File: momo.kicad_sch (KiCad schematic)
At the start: 97 parts, among them SW1 MX_SW_HS, SW10 MX_SW_HS, SW11 MX_SW_HS, SW12 MX_SW_HS, SW13 MX_SW_HS, SW14 MX_SW_HS, SW15 MX_SW_HS, SW16 MX_SW_HS, SW17 MX_SW_HS, SW18 MX_SW_HS, SW19 MX_SW_HS, SW2 MX_SW_HS, SW20 MX_SW_HS, SW21 MX_SW_HS, SW22 MX_SW_HS, SW23 MX_SW_HS, SW24 MX_SW_HS, SW25 MX_SW_HS, SW26 MX_SW_HS, SW27 MX_SW_HS, SW28 MX_SW_HS, SW29 MX_SW_HS, SW3 MX_SW_HS, SW30 MX_SW_HS, SW31 MX_SW_HS, SW32 MX_SW_HS, SW33 MX_SW_HS, SW34 MX_SW_HS, SW35 MX_SW_HS, SW36 MX_SW_HS, SW37 MX_SW_HS, SW38 MX_SW_HS, SW39 MX_SW_HS, SW4 MX_SW_HS, SW40 MX_SW_HS, SW41 MX_SW_HS, SW42 MX_SW_HS, SW43 MX_SW_HS, SW44 MX_SW_HS, SW45 MX_SW_HS, SW46 MX_SW_HS, SW47 MX_SW_HS, SW48 MX_SW_HS, SW5 MX_SW_HS, SW6 MX_SW_HS, SW7 MX_SW_HS, SW8 MX_SW_HS, SW9 MX_SW_HS, U1 WeAct-RP2040-Pico

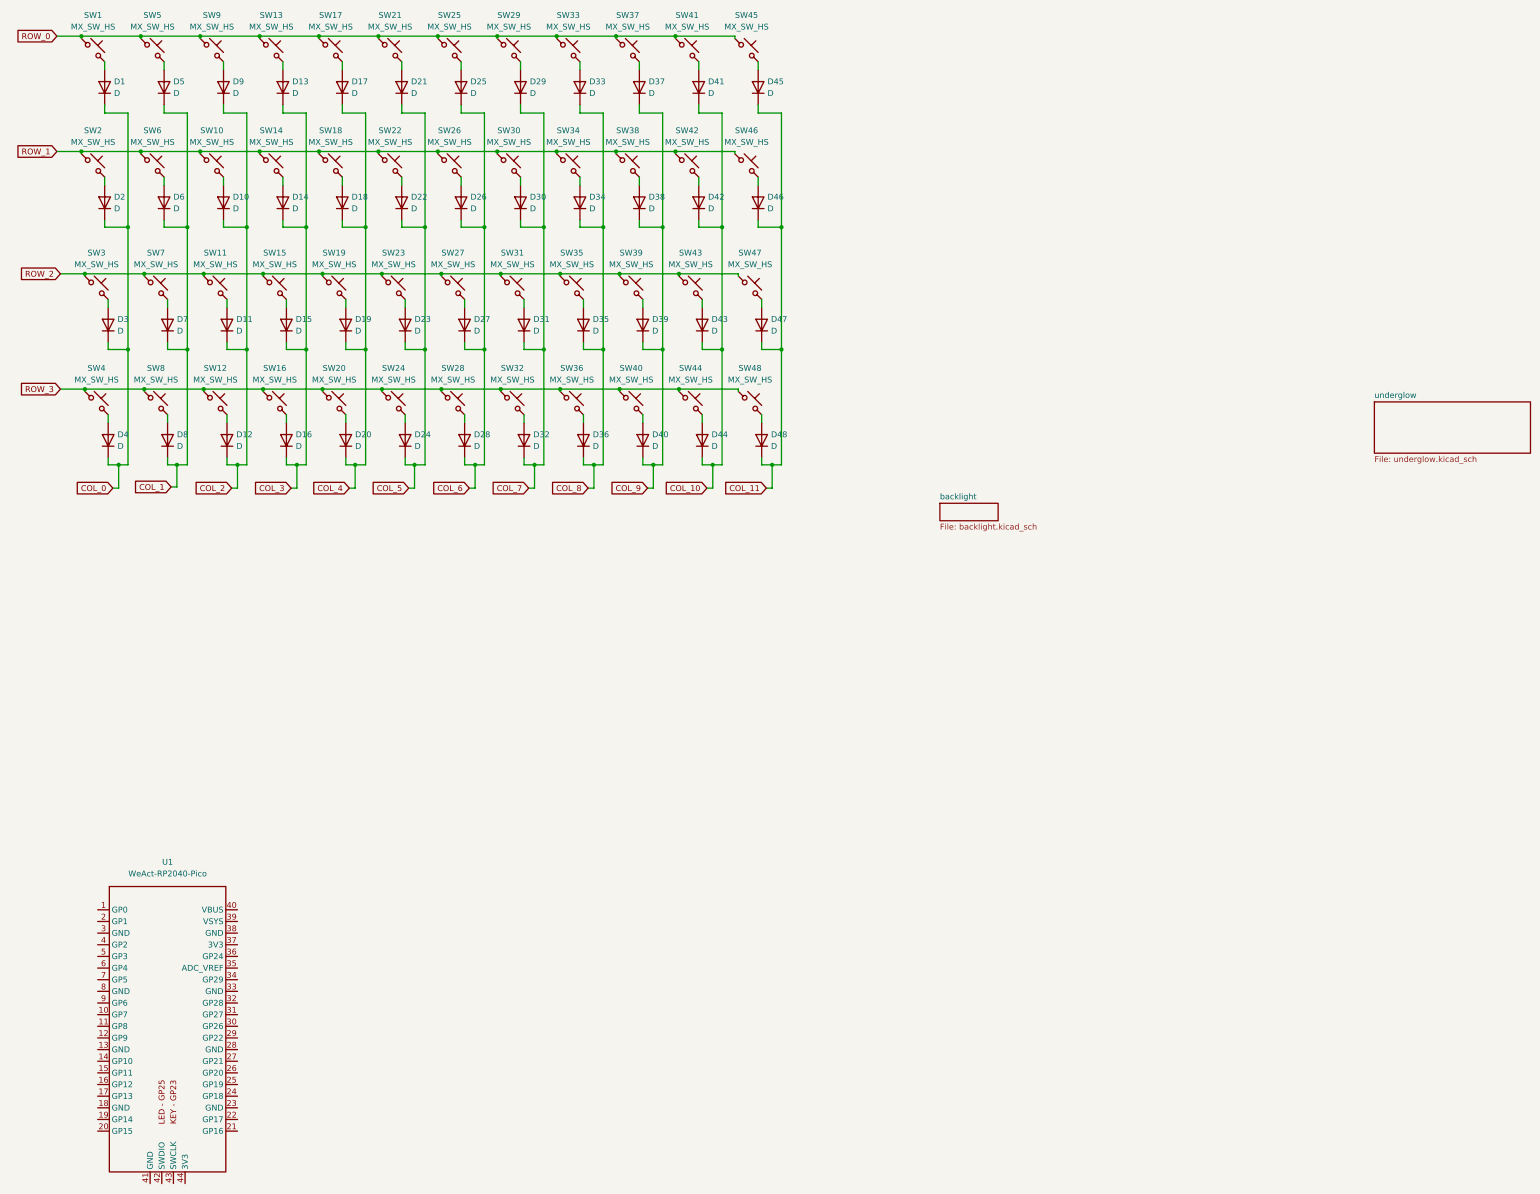
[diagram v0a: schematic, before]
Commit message: Pin wiring
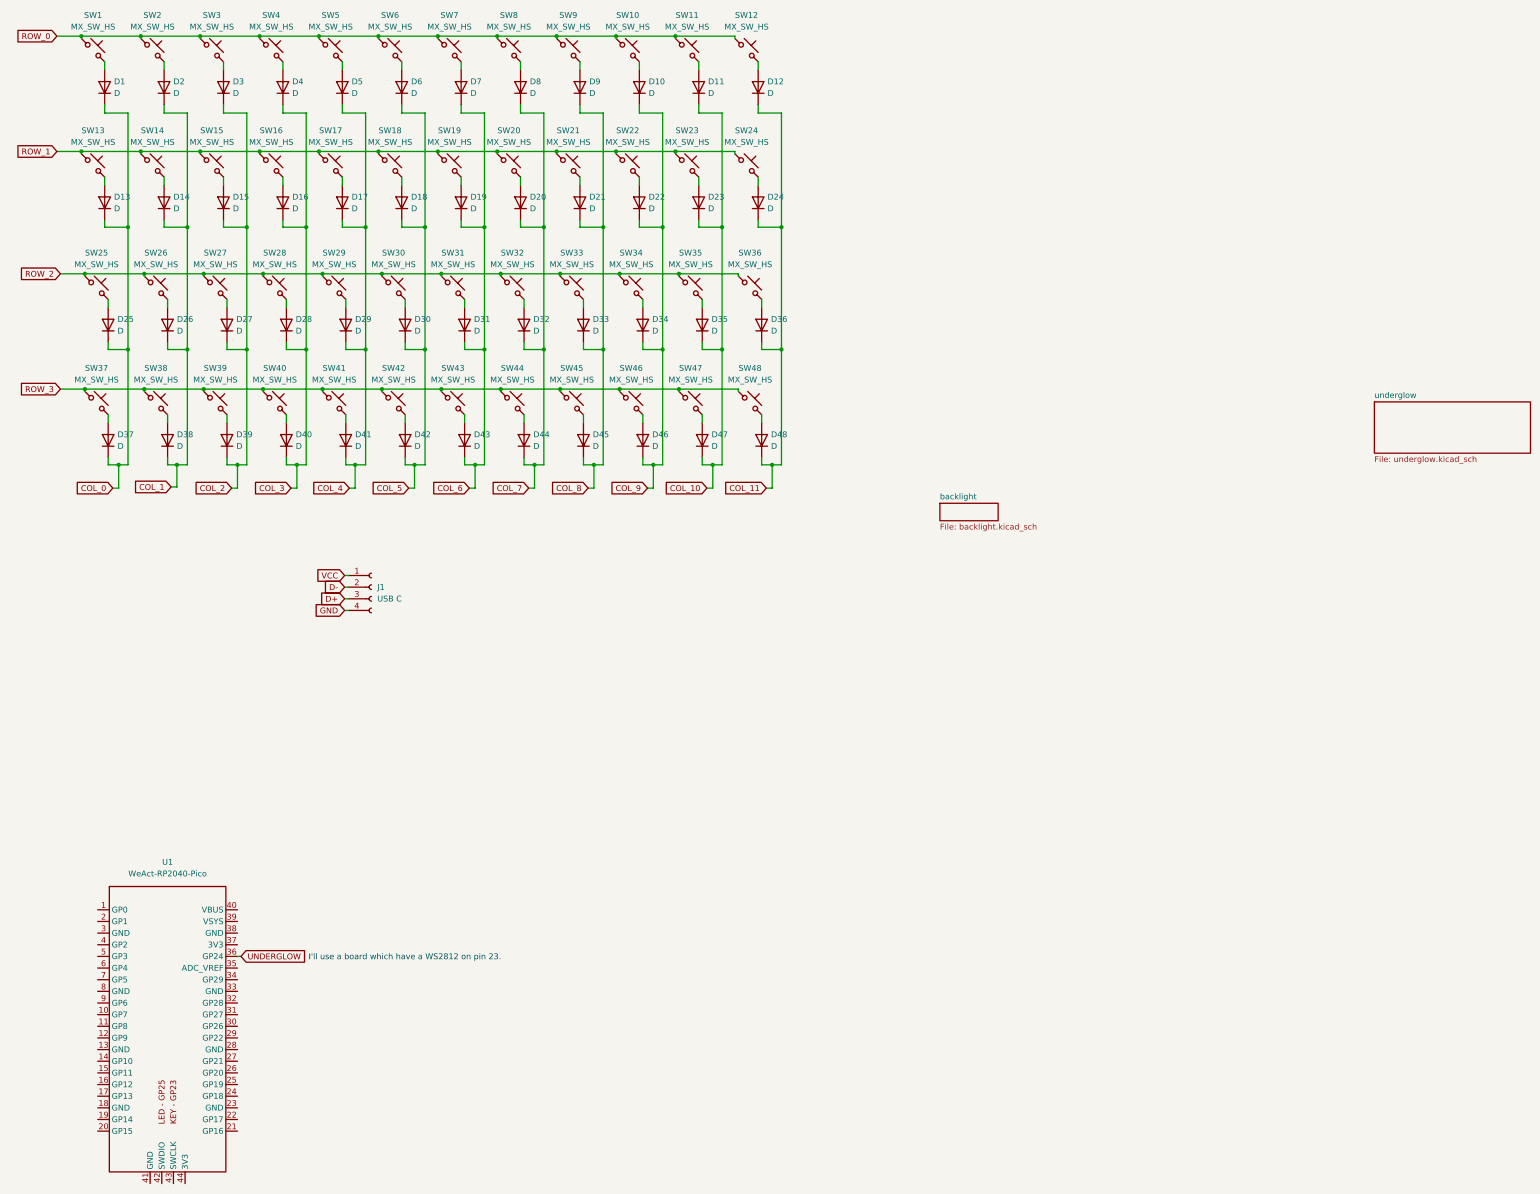
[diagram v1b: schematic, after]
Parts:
- added J1: USB C, Connector_PinHeader_2.54mm:PinHeader_1x04_P2.54mm_Vertical, symbol Connector:Conn_01x04_Female
- renumbered D37 to D10, D41 to D11, D45 to D12, D2 to D13, D6 to D14, D10 to D15, D14 to D16, D18 to D17, D22 to D18, D26 to D19, D5 to D2, D30 to D20, D34 to D21, D38 to D22, D42 to D23, D46 to D24, D3 to D25, D7 to D26, D11 to D27, D15 to D28, D19 to D29, D9 to D3, D23 to D30, D27 to D31, D31 to D32, D35 to D33, D39 to D34, D43 to D35, D47 to D36, D4 to D37, D8 to D38, D12 to D39, D13 to D4, D16 to D40, D20 to D41, D24 to D42, D28 to D43, D32 to D44, D36 to D45, D40 to D46, D44 to D47, D17 to D5, D21 to D6, D25 to D7, D29 to D8, D33 to D9, SW37 to SW10, SW41 to SW11, SW45 to SW12, SW2 to SW13, SW6 to SW14, SW10 to SW15, SW14 to SW16, SW18 to SW17, SW22 to SW18, SW26 to SW19, SW5 to SW2, SW30 to SW20, SW34 to SW21, SW38 to SW22, SW42 to SW23, SW46 to SW24, SW3 to SW25, SW7 to SW26, SW11 to SW27, SW15 to SW28, SW19 to SW29, SW9 to SW3, SW23 to SW30, SW27 to SW31, SW31 to SW32, SW35 to SW33, SW39 to SW34, SW43 to SW35, SW47 to SW36, SW4 to SW37, SW8 to SW38, SW12 to SW39, SW13 to SW4, SW16 to SW40, SW20 to SW41, SW24 to SW42, SW28 to SW43, SW32 to SW44, SW36 to SW45, SW40 to SW46, SW44 to SW47, SW17 to SW5, SW21 to SW6, SW25 to SW7, SW29 to SW8, SW33 to SW9
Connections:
- net UNDERGLOW: now reaches U1.36 (GP24)
- new net D+: J1.3 (Pin_3)
- new net D-: J1.2 (Pin_2)
- new net GND: J1.4 (Pin_4)
- new net VCC: J1.1 (Pin_1)
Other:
- note added: "I'll use a board which have a WS2812 on pin 23."
